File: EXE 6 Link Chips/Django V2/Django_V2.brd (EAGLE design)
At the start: 30.3 x 23.4 mm, 1 part

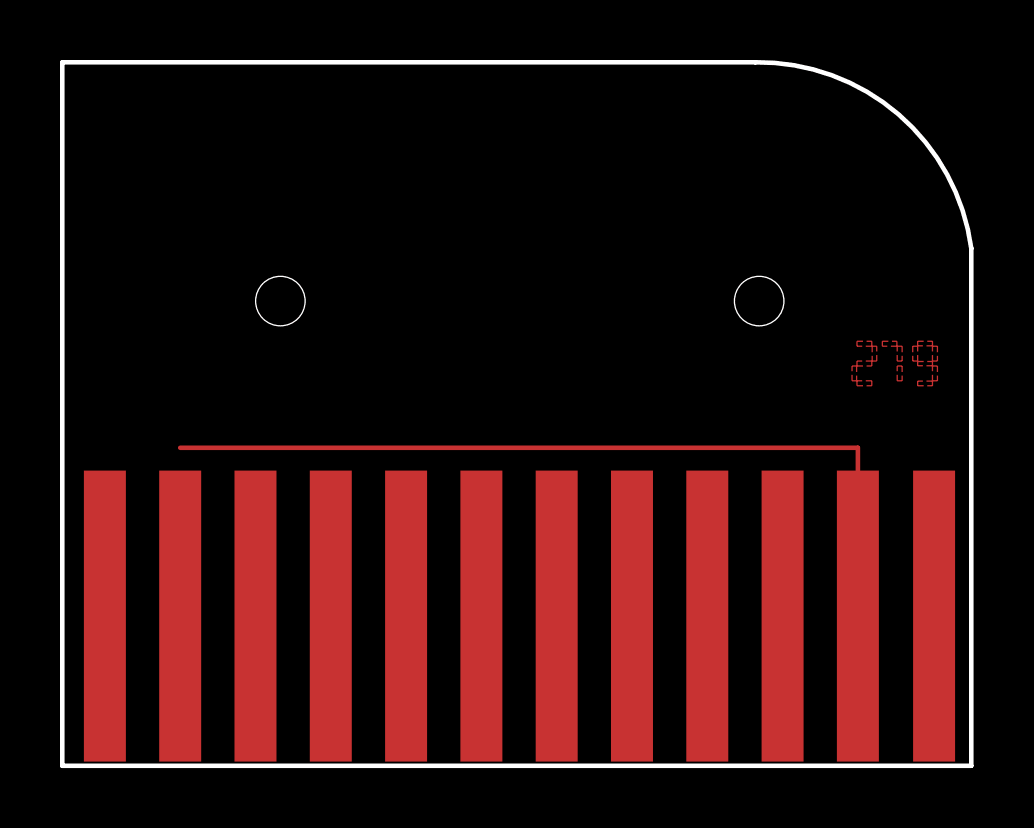
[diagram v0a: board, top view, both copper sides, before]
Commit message: Replace Django_V2.brd
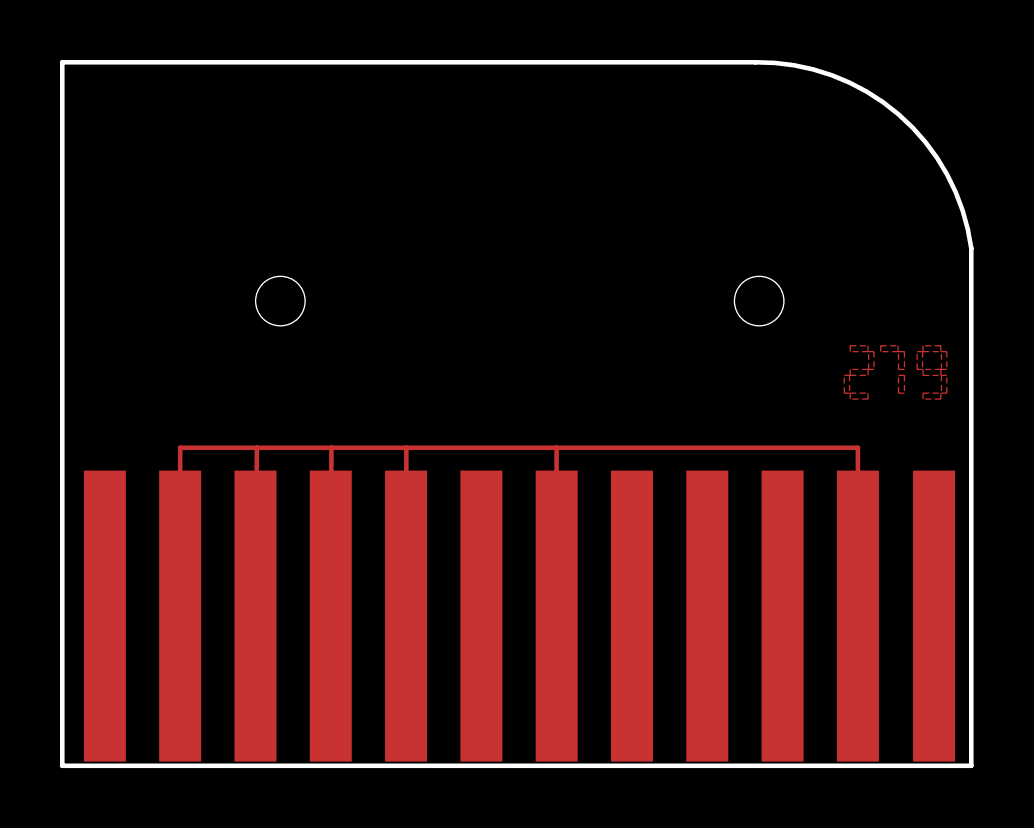
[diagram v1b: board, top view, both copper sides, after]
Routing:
- net N$1: track 28.2 -> 56.3 mm
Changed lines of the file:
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@@
 <setting verticaltext="up"/>
 </settings>
-<grid distance="1" unitdist="mic" unit="mic" style="dots" multiple="1" display="no" altdistance="1" altunitdist="mil" altunit="mm"/>
+<grid distance="1" unitdist="mic" unit="mm" style="dots" multiple="1" display="no" altdistance="1" altunitdist="mil" altunit="mm"/>
 <layers>
 <layer number="1" name="Top" color="4" fill="1" visible="yes" active="yes"/>
@@
 <contactref element="U$1" pad="P$11"/>
 <wire x1="56.72" y1="28.4" x2="56.72" y2="22.79" width="0.1524" layer="1"/>
-<wire x1="34.13" y1="28.4" x2="56.72" y2="28.4" width="0.1524" layer="1"/>
+<wire x1="34.13" y1="28.4" x2="36.687" y2="28.4" width="0.1524" layer="1"/>
 <contactref element="U$1" pad="P$2"/>
 <contactref element="U$1" pad="P$3"/>
@@
 <contactref element="U$1" pad="P$5"/>
 <contactref element="U$1" pad="P$7"/>
-<wire x1="41.66" y1="22.79" x2="46.68" y2="22.79" width="0" layer="19" extent="1-1"/>
-<wire x1="39.15" y1="22.79" x2="41.66" y2="22.79" width="0" layer="19" extent="1-1"/>
-<wire x1="36.64" y1="22.79" x2="39.15" y2="22.79" width="0" layer="19" extent="1-1"/>
-<wire x1="34.13" y1="22.79" x2="36.64" y2="22.79" width="0" layer="19" extent="1-1"/>
-<wire x1="34.13" y1="28.4" x2="34.13" y2="22.79" width="0" layer="19" extent="1-1"/>
+<wire x1="36.687" y1="28.4" x2="39.172" y2="28.4" width="0.1524" layer="1"/>
+<wire x1="39.172" y1="28.4" x2="41.669" y2="28.4" width="0.1524" layer="1"/>
+<wire x1="41.669" y1="28.4" x2="46.677" y2="28.4" width="0.1524" layer="1"/>
+<wire x1="46.677" y1="28.4" x2="56.72" y2="28.4" width="0.1524" layer="1"/>
+<wire x1="34.13" y1="22.79" x2="34.13" y2="28.4" width="0.1524" layer="1"/>
+<wire x1="36.64" y1="22.79" x2="36.687" y2="28.4" width="0.1524" layer="1"/>
+<wire x1="39.15" y1="22.79" x2="39.172" y2="28.4" width="0.1524" layer="1"/>
+<wire x1="41.66" y1="22.79" x2="41.669" y2="28.4" width="0.1524" layer="1"/>
+<wire x1="46.68" y1="22.79" x2="46.677" y2="28.4" width="0.1524" layer="1"/>
+</signal>
+<signal name="N$7">
+<polygon width="0.001" layer="1" rank="0">
+<vertex x="56.442409375" y="30.221"/>
+<vertex x="56.267740625" y="30.221"/>
+<vertex x="56.267740625" y="30.81398125"/>
+<vertex x="56.442409375" y="30.81398125"/>
+</polygon>
+</signal>
+<signal name="N$4">
+<polygon width="0.001" layer="1" rank="0">
+<vertex x="57.0584" y="30.02331875"/>
+<vertex x="56.465409375" y="30.02331875"/>
+<vertex x="56.465409375" y="30.221"/>
+<vertex x="57.0584" y="30.221"/>
+</polygon>
+</signal>
+<signal name="N$3">
+<polygon width="0.001" layer="1" rank="0">
+<vertex x="56.465409375" y="31.01165"/>
+<vertex x="56.465409375" y="30.81398125"/>
+<vertex x="57.0584" y="30.81398125"/>
+<vertex x="57.0584" y="31.01165"/>
+</polygon>
+</signal>
+<signal name="N$2">
+<polygon width="0.001" layer="1" rank="0">
+<vertex x="57.25608125" y="31.01165"/>
+<vertex x="57.0774" y="31.01165"/>
+<vertex x="57.0774" y="31.60465"/>
+<vertex x="57.25608125" y="31.60465"/>
+</polygon>
+</signal>
+<signal name="N$18">
+<polygon width="0.001" layer="1" rank="0">
+<vertex x="57.0584" y="31.60465"/>
+<vertex x="56.465409375" y="31.60465"/>
+<vertex x="56.465409375" y="31.802309375"/>
+<vertex x="57.0584" y="31.802309375"/>
+</polygon>
+</signal>
+<signal name="N$21">
+<polygon width="0.001" layer="1" rank="0">
+<vertex x="58.27206875" y="30.221"/>
+<vertex x="58.0744" y="30.221"/>
+<vertex x="58.0744" y="30.81398125"/>
+<vertex x="58.27206875" y="30.81398125"/>
+</polygon>
 </signal>
 <signal name="N$5">
 <polygon width="0.001" layer="1" rank="0">
-<vertex x="56.689509375" y="30.6325"/>
-<vertex x="56.689509375" y="30.46776875"/>
-<vertex x="57.18366875" y="30.46776875"/>
-<vertex x="57.18366875" y="30.6325"/>
-</polygon>
-</signal>
-<signal name="N$4">
-<polygon width="0.001" layer="1" rank="0">
-<vertex x="56.677509375" y="30.6325"/>
-<vertex x="56.52478125" y="30.6325"/>
-<vertex x="56.52478125" y="31.12665"/>
-<vertex x="56.677509375" y="31.12665"/>
-</polygon>
-</signal>
-<signal name="N$3">
-<polygon width="0.001" layer="1" rank="0">
-<vertex x="56.689509375" y="31.29138125"/>
-<vertex x="56.689509375" y="31.12665"/>
-<vertex x="57.18366875" y="31.12665"/>
-<vertex x="57.18366875" y="31.29138125"/>
-</polygon>
-</signal>
-<signal name="N$2">
-<polygon width="0.001" layer="1" rank="0">
-<vertex x="57.19666875" y="31.785540625"/>
-<vertex x="57.19666875" y="31.29138125"/>
-<vertex x="57.3484" y="31.29138125"/>
-<vertex x="57.3484" y="31.785540625"/>
-</polygon>
-</signal>
-<signal name="N$18">
-<polygon width="0.001" layer="1" rank="0">
-<vertex x="57.18366875" y="31.785540625"/>
-<vertex x="56.689509375" y="31.785540625"/>
-<vertex x="56.689509375" y="31.950259375"/>
-<vertex x="57.18366875" y="31.950259375"/>
-</polygon>
-</signal>
-<signal name="N$21">
-<polygon width="0.001" layer="1" rank="0">
-<vertex x="58.195059375" y="30.6325"/>
-<vertex x="58.030340625" y="30.6325"/>
-<vertex x="58.030340625" y="31.12665"/>
-<vertex x="58.195059375" y="31.12665"/>
+<vertex x="58.0604" y="31.60465"/>
+<vertex x="57.481409375" y="31.60465"/>
+<vertex x="57.481409375" y="31.802309375"/>
+<vertex x="58.0604" y="31.802309375"/>
+</polygon>
+</signal>
+<signal name="N$25">
+<polygon width="0.001" layer="1" rank="0">
+<vertex x="58.27206875" y="31.01165"/>
+<vertex x="58.0744" y="31.01165"/>
+<vertex x="58.0744" y="31.60465"/>
+<vertex x="58.27206875" y="31.60465"/>
+</polygon>
+</signal>
+<signal name="N$11">
+<polygon width="0.001" layer="1" rank="0">
+<vertex x="59.50575" y="30.81398125"/>
+<vertex x="59.50575" y="30.221"/>
+<vertex x="59.683409375" y="30.221"/>
+<vertex x="59.683409375" y="30.81398125"/>
+</polygon>
+</signal>
+<signal name="N$10">
+<polygon width="0.001" layer="1" rank="0">
+<vertex x="59.48575" y="30.02331875"/>
+<vertex x="58.892759375" y="30.02331875"/>
+<vertex x="58.892759375" y="30.221"/>
+<vertex x="59.48575" y="30.221"/>
+</polygon>
+</signal>
+<signal name="N$9">
+<polygon width="0.001" layer="1" rank="0">
+<vertex x="58.892759375" y="31.01165"/>
+<vertex x="58.892759375" y="30.81398125"/>
+<vertex x="59.48575" y="30.81398125"/>
+<vertex x="59.48575" y="31.01165"/>
+</polygon>
+</signal>
+<signal name="N$8">
+<polygon width="0.001" layer="1" rank="0">
+<vertex x="59.683409375" y="31.01165"/>
+<vertex x="59.50475" y="31.01165"/>
+<vertex x="59.50475" y="31.60465"/>
+<vertex x="59.683409375" y="31.60465"/>
 </polygon>
 </signal>
 <signal name="N$6">
 <polygon width="0.001" layer="1" rank="0">
-<vertex x="58.020340625" y="31.785540625"/>
-<vertex x="57.53618125" y="31.785540625"/>
-<vertex x="57.53618125" y="31.950259375"/>
-<vertex x="58.020340625" y="31.950259375"/>
-</polygon>
-</signal>
-<signal name="N$25">
-<polygon width="0.001" layer="1" rank="0">
-<vertex x="58.195059375" y="31.29138125"/>
-<vertex x="58.030340625" y="31.29138125"/>
-<vertex x="58.030340625" y="31.785540625"/>
-<vertex x="58.195059375" y="31.785540625"/>
-</polygon>
-</signal>
-<signal name="N$10">
-<polygon width="0.001" layer="1" rank="0">
-<vertex x="58.7123" y="30.6225"/>
-<vertex x="58.7123" y="30.46776875"/>
-<vertex x="59.206459375" y="30.46776875"/>
-<vertex x="59.206459375" y="30.6225"/>
-</polygon>
-</signal>
-<signal name="N$11">
-<polygon width="0.001" layer="1" rank="0">
-<vertex x="59.37118125" y="30.6325"/>
-<vertex x="59.206459375" y="30.6325"/>
-<vertex x="59.206459375" y="31.12665"/>
-<vertex x="59.37118125" y="31.12665"/>
-</polygon>
-</signal>
-<signal name="N$9">
-<polygon width="0.001" layer="1" rank="0">
-<vertex x="59.206459375" y="31.13465"/>
-<vertex x="58.7123" y="31.13465"/>
-<vertex x="58.7123" y="31.27638125"/>
-<vertex x="59.206459375" y="31.27638125"/>
-</polygon>
-</signal>
-<signal name="N$8">
-<polygon width="0.001" layer="1" rank="0">
-<vertex x="59.37118125" y="31.29138125"/>
-<vertex x="59.206459375" y="31.29138125"/>
-<vertex x="59.206459375" y="31.785540625"/>
-<vertex x="59.37118125" y="31.785540625"/>
-</polygon>
-</signal>
-<signal name="N$7">
-<polygon width="0.001" layer="1" rank="0">
-<vertex x="58.54756875" y="31.785540625"/>
-<vertex x="58.54756875" y="31.29138125"/>
-<vertex x="58.7123" y="31.29138125"/>
-<vertex x="58.7123" y="31.785540625"/>
+<vertex x="58.892759375" y="31.802309375"/>
+<vertex x="58.892759375" y="31.60465"/>
+<vertex x="59.48575" y="31.60465"/>
+<vertex x="59.48575" y="31.802309375"/>
 </polygon>
 </signal>
 <signal name="N$37">
 <polygon width="0.001" layer="1" rank="0">
-<vertex x="59.206459375" y="31.798540625"/>
-<vertex x="58.7123" y="31.798540625"/>
-<vertex x="58.7123" y="31.950259375"/>
-<vertex x="59.206459375" y="31.950259375"/>
-</polygon>
-</signal>
+<vertex x="58.875759375" y="31.01165"/>
+<vertex x="58.695090625" y="31.01165"/>
+<vertex x="58.695090625" y="31.60465"/>
+<vertex x="58.875759375" y="31.60465"/>
+</polygon>
+</signal>
